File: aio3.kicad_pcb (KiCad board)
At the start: 2 copper layers, 64.3 x 38.1 mm, 24 parts, among them SW1 SW_Push, U1 ATmega32U4-AU, Y1 16MHz

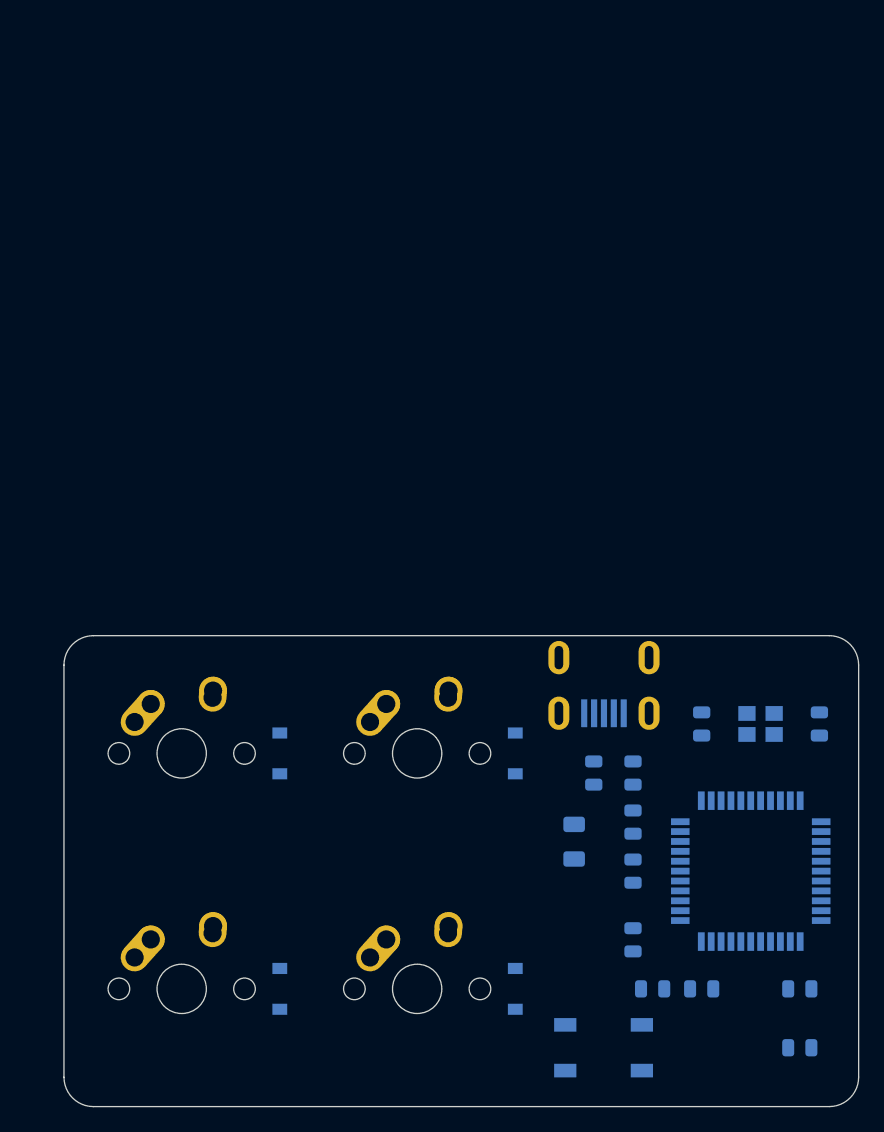
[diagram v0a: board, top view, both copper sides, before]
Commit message: Finished Board. Maybe.
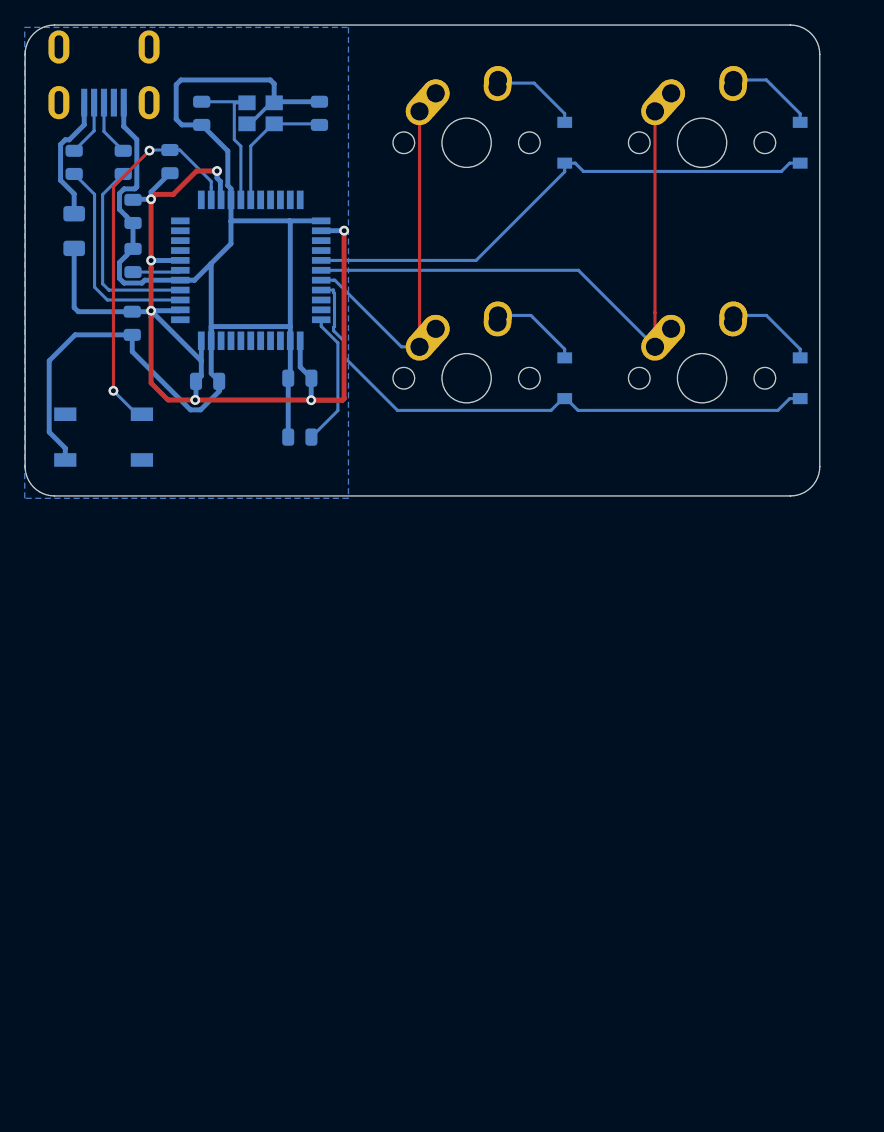
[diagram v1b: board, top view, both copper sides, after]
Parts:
- moved R3 77.5 mm to (87.9, 72.8), turned to 90 degrees
- moved R1 64.9 mm to (80.2, 72.8)
- moved R2 64.4 mm to (84.2, 72.8)
- moved C6 64.3 mm to (84.9, 85.9), turned to 270 degrees
- moved C7 63.8 mm to (85.0, 80.8)
- moved F1 63.8 mm to (80.2, 78.4)
- moved R4 63.8 mm to (98.5, 95.1)
- moved SW1 63.8 mm to (82.6, 95.1)
- moved USB1 63.8 mm to (82.6, 63.5)
- moved C1 63.8 mm to (85.0, 76.8)
- moved C2 63.8 mm to (98.5, 90.3)
- moved C4 63.8 mm to (100.0, 68.9)
- moved C5 63.8 mm to (90.5, 68.9)
- moved Y1 63.8 mm to (95.3, 68.9)
- moved C3 63.4 mm to (91.0, 90.6)
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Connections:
- U1 pad 27: Net-(U1-Pad27) -> ROW0
- U1 pad 28: Net-(U1-Pad28) -> COL1
- U1 pad 29: Net-(U1-Pad29) -> COL0
- U1 pad 30: Net-(U1-Pad30) -> ROW1
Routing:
- net GND: track 0.00 -> 129.8 mm
- net +5V: track 0.00 -> 92.6 mm, vias 0 -> 7
- net COL1: track 0.00 -> 48.6 mm
- net ROW1: track 0.00 -> 46.7 mm
- net ROW0: track 0.00 -> 43.0 mm
- net Net-(R3-Pad2): track 0.00 -> 31.3 mm, vias 0 -> 2
- net COL0: track 0.00 -> 29.2 mm
- net Net-(R1-Pad1): track 0.00 -> 17.2 mm
- net Net-(R2-Pad1): track 0.00 -> 16.1 mm
- net Net-(C5-Pad1): track 0.00 -> 12.7 mm
- net Net-(R4-Pad2): track 0.00 -> 10.9 mm
- net Net-(C4-Pad1): track 0.00 -> 10.7 mm
- net VCC: track 0.00 -> 10.4 mm
- net Net-(D2-Pad2): track 0.00 -> 6.09 mm
- net Net-(D4-Pad2): track 0.00 -> 6.09 mm
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- added copper zone on B.Cu, net GND
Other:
- net class Power added: clearance 0.2, trace_width 0.4, via_dia 0.8, via_drill 0.4
